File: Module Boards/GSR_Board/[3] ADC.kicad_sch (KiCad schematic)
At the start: 15 parts, among them U7 LTC1864LIMS8#PBF, U8 TXB0104RUTR, U9 TPS22916CYFPR

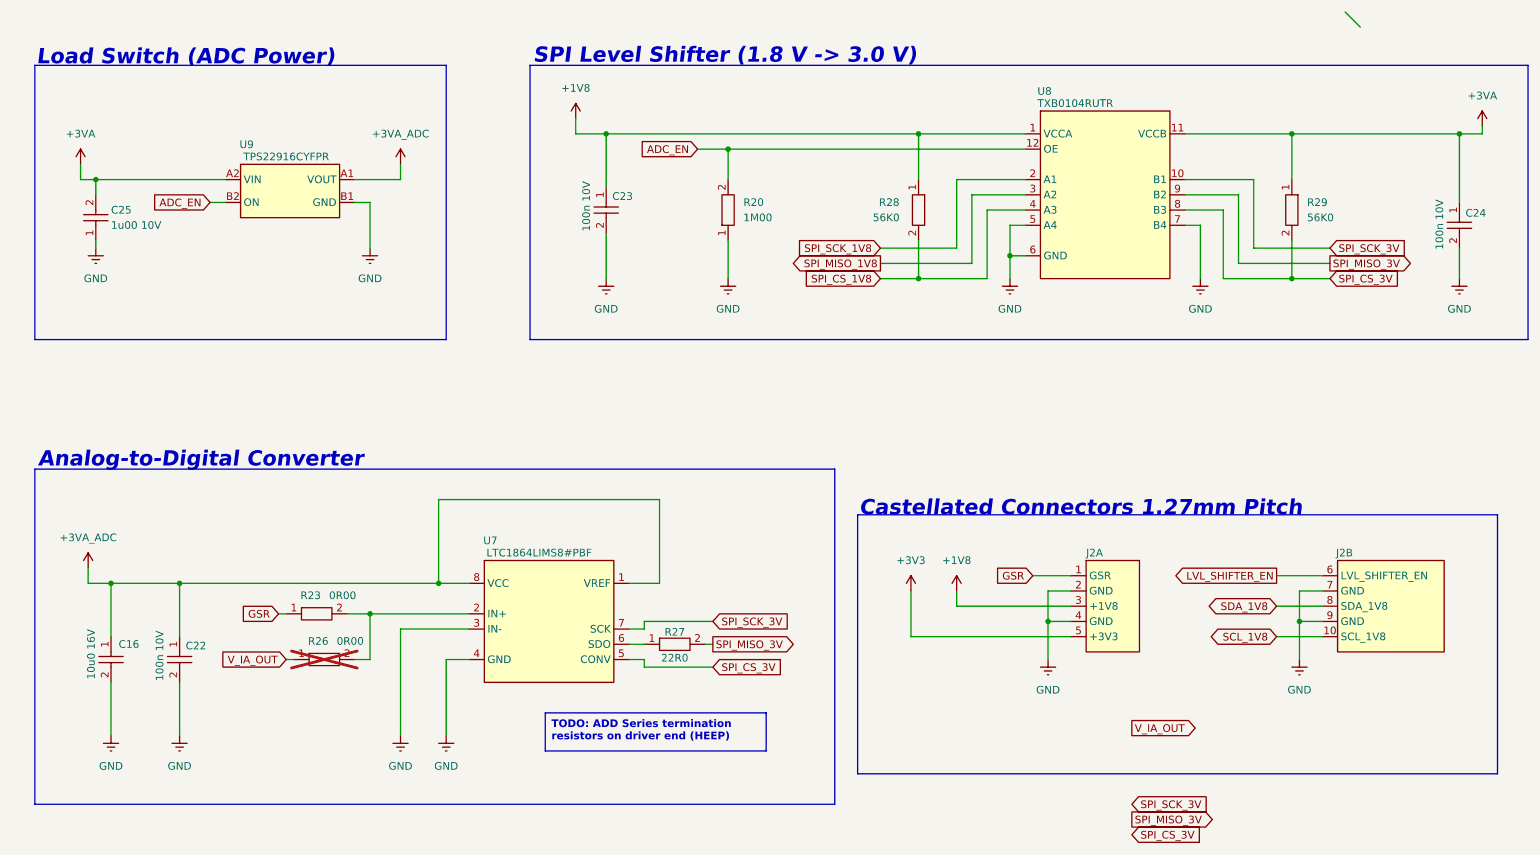
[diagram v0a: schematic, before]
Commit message: Finished Routing of GSR Board
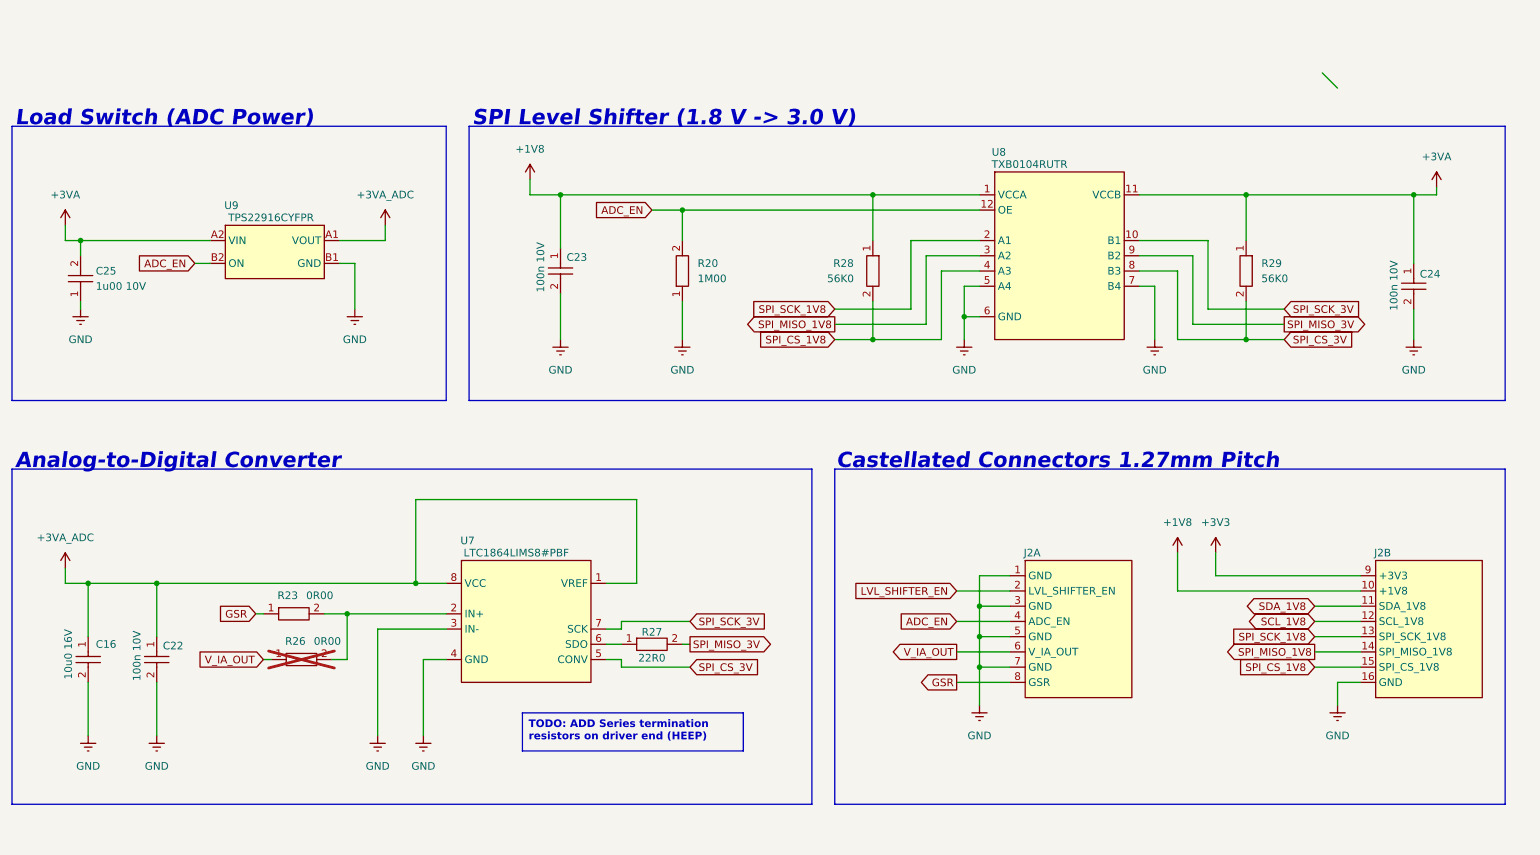
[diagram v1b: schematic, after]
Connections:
- net +1V8: now also J2.10 (+1V8); no longer J2.3 (+1V8)
- net +3V3: now also J2.9 (+3V3); no longer J2.5 (+3V3)
- net ADC_EN: now also J2.4 (ADC_EN)
- net GND: now also J2.1 (GND), J2.16 (GND), J2.3 (GND), J2.5 (GND), J2.7 (GND); no longer J2.2 (GND), J2.4 (GND), J2.7 (GND), J2.9 (GND)
- net GSR: now also J2.8 (GSR); no longer J2.1 (GSR)
- net LVL_SHIFTER_EN: now also J2.2 (LVL_SHIFTER_EN); no longer J2.6 (LVL_SHIFTER_EN)
- net SCL_1V8: now also J2.12 (SCL_1V8); no longer J2.10 (SCL_1V8)
- net SDA_1V8: now also J2.11 (SDA_1V8); no longer J2.8 (SDA_1V8)
- net SPI_CS_1V8: now also J2.15 (SPI_CS_1V8)
- net SPI_MISO_1V8: now also J2.14 (SPI_MISO_1V8)
- net SPI_SCK_1V8: now also J2.13 (SPI_SCK_1V8)
- net V_IA_OUT: now also J2.6 (V_IA_OUT)
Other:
- moved on the sheet: C16, C22, C23, C24, C25, R20, R23, R26, R27, R28, R29, U7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
